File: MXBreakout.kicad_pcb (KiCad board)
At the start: 2 copper layers, 41.2 x 21.2 mm, 18 parts, among them U1 Wii-MX, Y1 32.768kHz

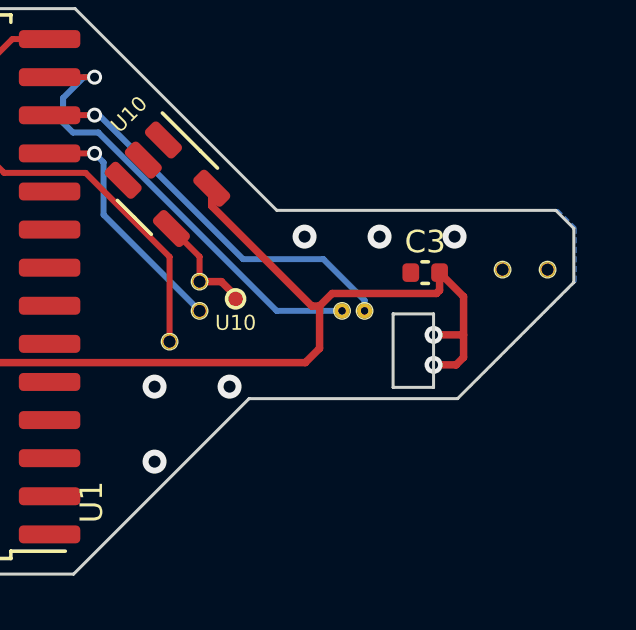
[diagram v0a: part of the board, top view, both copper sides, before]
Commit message: Minor track tidy
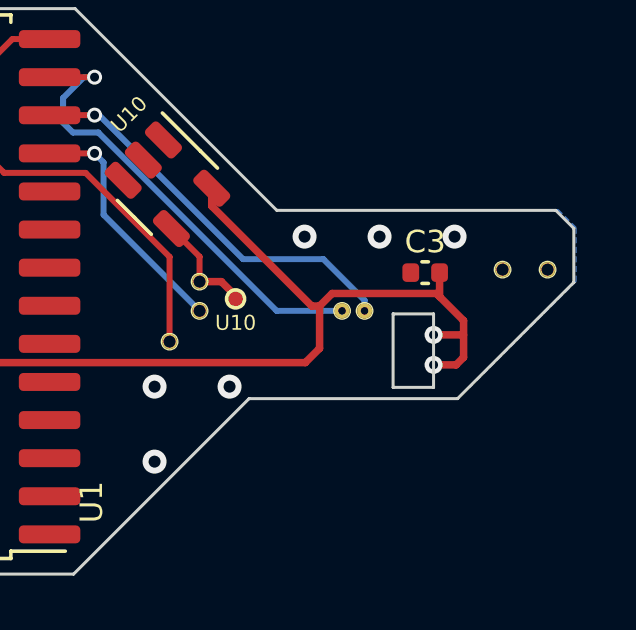
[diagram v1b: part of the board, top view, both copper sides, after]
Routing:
- net +3.3V: track 52.6 -> 52.0 mm
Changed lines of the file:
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@@
 	)
 	(segment
-		(start 82.8 53.525)
-		(end 82.8 55.55)
+		(start 81.895 53.42)
+		(end 82.8 54.325)
 		(width 0.25)
 		(layer "F.Cu")
@@
 		(start 60.55 57.025)
 		(end 60.55 59.260908)
+		(width 0.25)
+		(layer "F.Cu")
+		(net 11)
+	)
+	(segment
+		(start 82.8 54.325)
+		(end 82.8 55.55)
 		(width 0.25)
 		(layer "F.Cu")
@@
 		(start 58.7 57.025)
 		(end 58.7 57.64)
+		(width 0.25)
+		(layer "F.Cu")
+		(net 11)
+	)
+	(segment
+		(start 82.55 55.8)
+		(end 82 55.8)
 		(width 0.25)
 		(layer "F.Cu")
@@
 	)
 	(segment
-		(start 82 52.725)
-		(end 82 53.315)
-		(width 0.25)
-		(layer "F.Cu")
-		(net 11)
-	)
-	(segment
 		(start 82.8 55.55)
 		(end 82.55 55.8)
-		(width 0.25)
-		(layer "F.Cu")
-		(net 11)
-	)
-	(segment
-		(start 82 53.315)
-		(end 81.895 53.42)
 		(width 0.25)
 		(layer "F.Cu")
@@
 		(start 59.2 47.48)
 		(end 60.224999 47.48)
+		(width 0.25)
+		(layer "F.Cu")
+		(net 11)
+	)
+	(segment
+		(start 82 52.725)
+		(end 82 53.525)
 		(width 0.25)
 		(layer "F.Cu")
@@
 	)
 	(segment
-		(start 82.55 55.8)
-		(end 82 55.8)
-		(width 0.25)
-		(layer "F.Cu")
-		(net 11)
-	)
-	(segment
 		(start 59.630908 60.18)
 		(end 59.2 60.18)
@@
 		(width 0.25)
 		(layer "F.Cu")
-		(net 11)
-	)
-	(segment
-		(start 82 52.725)
-		(end 82.8 53.525)
-		(width 0.25)
-		(layer "F.Cu")
